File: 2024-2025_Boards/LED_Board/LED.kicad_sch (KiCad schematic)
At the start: 11 parts, among them J5 Conn_01x05_Pin, U5 CSD88537ND, U6 CSD88537ND

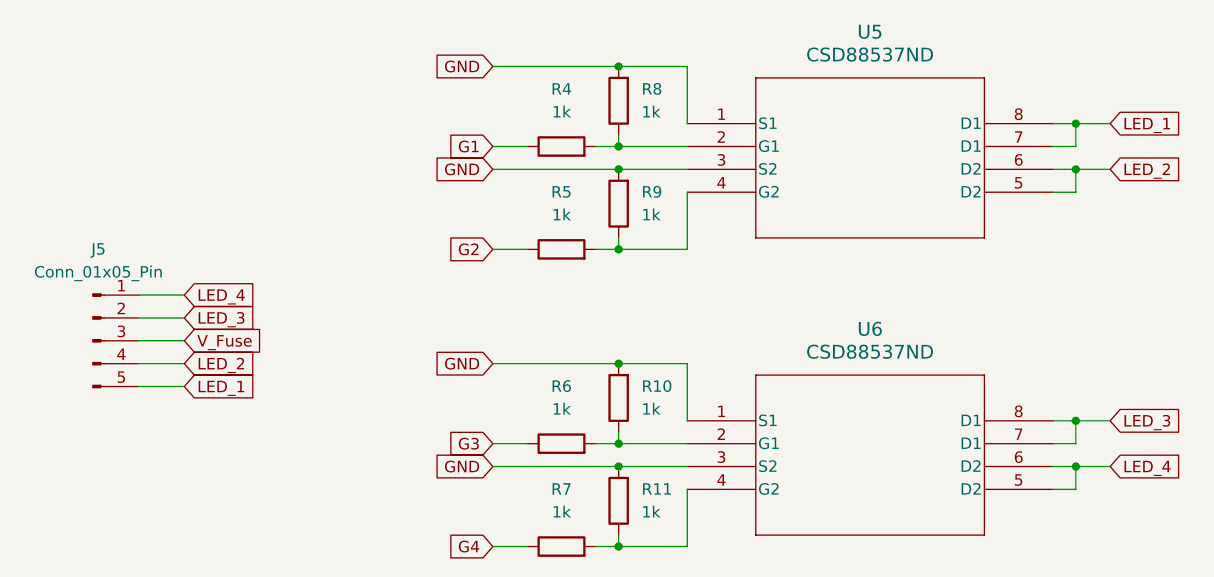
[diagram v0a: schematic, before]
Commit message: Pins on correct side
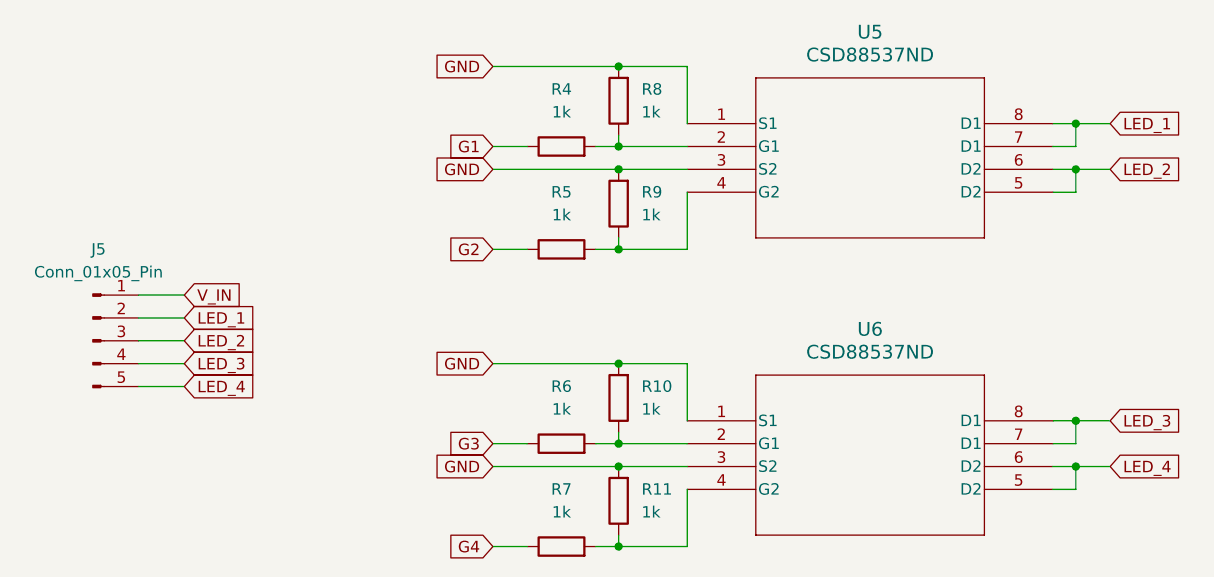
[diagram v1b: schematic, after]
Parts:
- J5: footprint Cornell_Mars_Rover:CONN05_GRPB051VWCN-RC_SUL -> Connector_JST:JST_EH_S5B-EH_1x05_P2.50mm_Horizontal
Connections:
- net V_Fuse is gone; now on net LED_2: J5.3 (Pin_3)
- net LED_1: now also J5.2 (Pin_2); no longer J5.5 (Pin_5)
- net LED_2: no longer J5.4 (Pin_4)
- net LED_3: now also J5.4 (Pin_4); no longer J5.2 (Pin_2)
- net LED_4: now also J5.5 (Pin_5); no longer J5.1 (Pin_1)
- new net V_IN: J5.1 (Pin_1)

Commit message: Board fixes
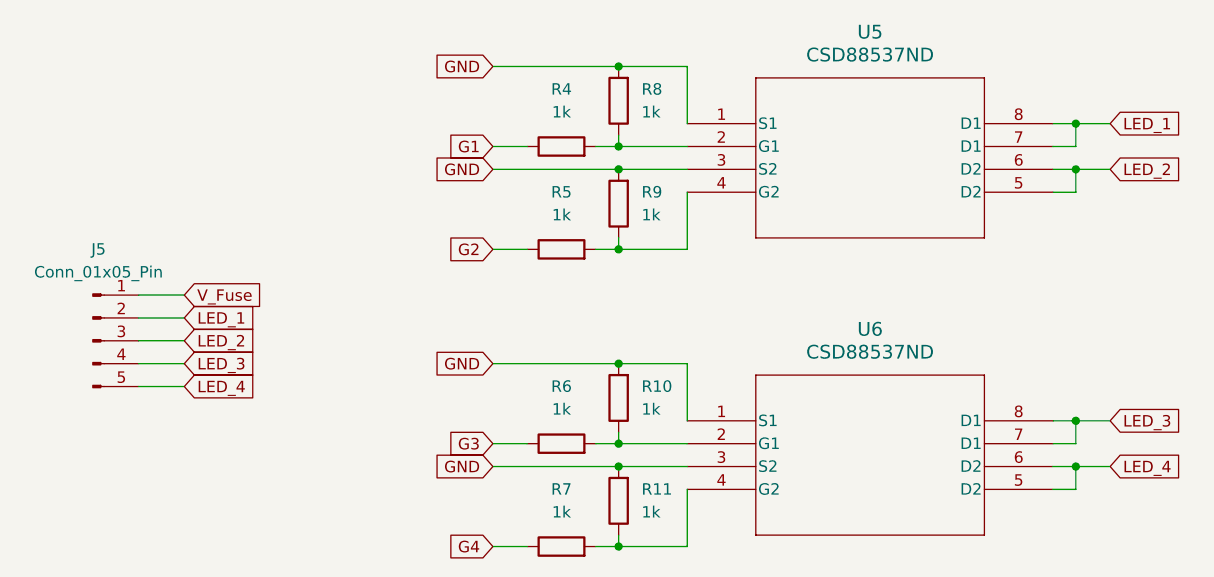
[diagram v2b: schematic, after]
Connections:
- net V_IN renamed V_Fuse
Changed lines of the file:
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@@
 		)
 	)
-	(global_label "V_IN"
+	(global_label "V_Fuse"
 		(shape input)
 		(at 90.17 90.17 0)
@@
 		)
 		(property "Intersheetrefs" "${INTERSHEET_REFS}"
-			(at 97.1467 90.17 0)
+			(at 99.5657 90.17 0)
 			(effects
 				(font

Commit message: Symbol library fix
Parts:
- U5, U6: footprint Cornell_Mars_Rover:CSD88537ND8-M -> D8; symbol CMR_N_Channel_Power_Mosfet:CSD88537ND -> Cornell_Mars_Rover:CSD88537ND
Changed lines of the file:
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@@
 	)
 	(symbol
-		(lib_id "CMR_N_Channel_Power_Mosfet:CSD88537ND")
+		(lib_id "Cornell_Mars_Rover:CSD88537ND")
 		(at 146.05 104.14 0)
 		(unit 1)
@@
 			)
 		)
-		(property "Footprint" "Cornell_Mars_Rover:CSD88537ND8-M"
+		(property "Footprint" "D8"
 			(at 146.05 104.14 0)
 			(effects
@@
 	)
 	(symbol
-		(lib_id "CMR_N_Channel_Power_Mosfet:CSD88537ND")
+		(lib_id "Cornell_Mars_Rover:CSD88537ND")
 		(at 146.05 71.12 0)
 		(unit 1)
@@
 			)
 		)
-		(property "Footprint" "Cornell_Mars_Rover:CSD88537ND8-M"
+		(property "Footprint" "D8"
 			(at 146.05 71.12 0)
 			(effects
